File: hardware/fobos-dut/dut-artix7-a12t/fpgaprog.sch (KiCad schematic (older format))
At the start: 6 parts, among them U1 XC7A12T-CSG325

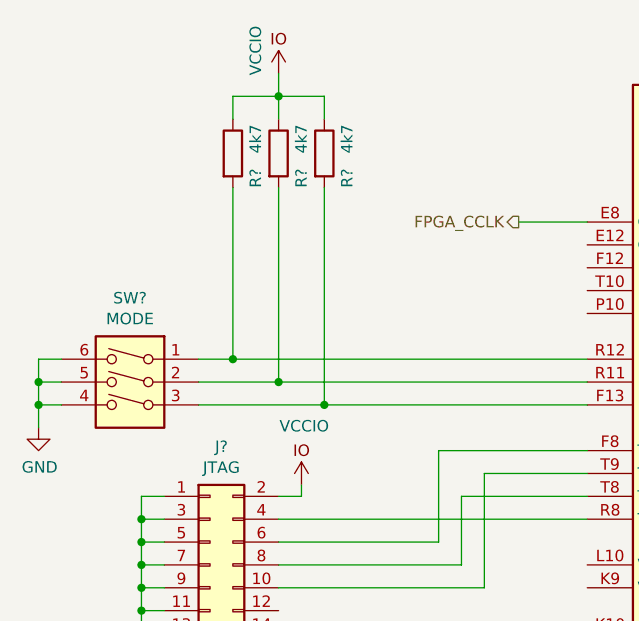
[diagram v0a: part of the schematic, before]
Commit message: artix 7 dut updates
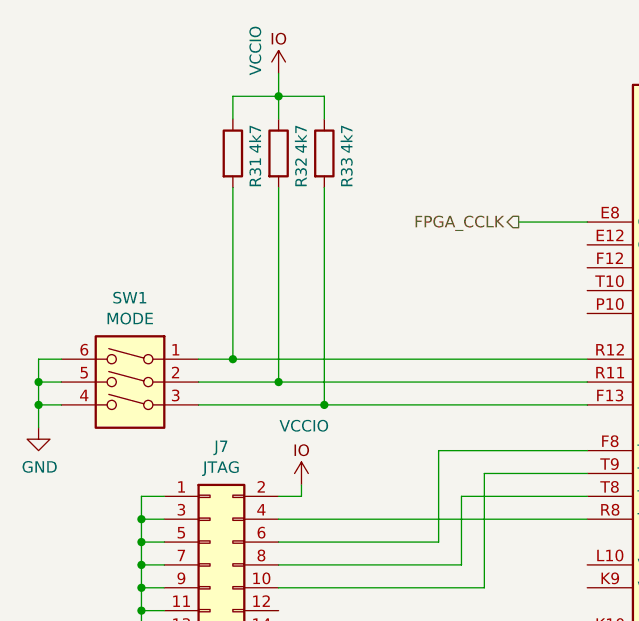
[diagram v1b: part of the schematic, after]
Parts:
- gave numbers to parts that had none: 5
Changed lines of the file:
@@
 $EndBitmap
 $Comp
-L Switch:SW_DIP_x03 SW?
+L Switch:SW_DIP_x03 SW1
 U 1 1 5F5037BE
 P 4500 3200
-F 0 "SW?" H 4500 3667 50  0000 C CNN
+F 0 "SW1" H 4500 3667 50  0000 C CNN
 F 1 "MODE" H 4500 3576 50  0000 C CNN
 F 2 "" H 4500 3200 50  0001 C CNN
@@
 $EndComp
 $Comp
-L power:GND #PWR?
+L power:GND #PWR0129
 U 1 1 5F505FAD
 P 4100 3300
-F 0 "#PWR?" H 4100 3050 50  0001 C CNN
+F 0 "#PWR0129" H 4100 3050 50  0001 C CNN
 F 1 "GND" H 4105 3127 50  0000 C CNN
 F 2 "" H 4100 3300 50  0001 C CNN
@@
 	4800 3200 5350 3200
 $Comp
-L Device:R R?
+L Device:R R33
 U 1 1 5F5112B7
 P 5350 2100
-F 0 "R?" V 5450 1950 50  0000 L CNN
+F 0 "R33" V 5450 1950 50  0000 L CNN
 F 1 "4k7" V 5450 2100 50  0000 L CNN
 F 2 "Resistor_SMD:R_0603_1608Metric" V 5280 2100 50  0001 C CNN
@@
 $EndComp
 $Comp
-L Device:R R?
+L Device:R R32
 U 1 1 5F518AC2
 P 5150 2100
-F 0 "R?" V 5250 1950 50  0000 L CNN
+F 0 "R32" V 5250 1950 50  0000 L CNN
 F 1 "4k7" V 5250 2100 50  0000 L CNN
 F 2 "Resistor_SMD:R_0603_1608Metric" V 5080 2100 50  0001 C CNN
@@
 $EndComp
 $Comp
-L Device:R R?
+L Device:R R31
 U 1 1 5F518EEF
 P 4950 2100
-F 0 "R?" V 5050 1950 50  0000 L CNN
+F 0 "R31" V 5050 1950 50  0000 L CNN
 F 1 "4k7" V 5050 2100 50  0000 L CNN
 F 2 "Resistor_SMD:R_0603_1608Metric" V 4880 2100 50  0001 C CNN
@@
 Connection ~ 5150 1850
 $Comp
-L cerg:VCCIO #PWR?
+L cerg:VCCIO #PWR0130
 U 1 1 5F520C1F
 P 5150 1750
-F 0 "#PWR?" H 5150 1600 50  0001 C CNN
+F 0 "#PWR0130" H 5150 1600 50  0001 C CNN
 F 1 "VCCIO" V 5050 1850 50  0000 C CNN
 F 2 "" H 5150 1750 50  0001 C CNN
@@
 	5150 1750 5150 1850
 $Comp
-L Connector_Generic:Conn_02x07_Odd_Even J?
+L Connector_Generic:Conn_02x07_Odd_Even J7
 U 1 1 5F5293C6
 P 4850 3900
-F 0 "J?" H 4900 4417 50  0000 C CNN
+F 0 "J7" H 4900 4417 50  0000 C CNN
 F 1 "JTAG" H 4900 4326 50  0000 C CNN
 F 2 "" H 4850 3900 50  0001 C CNN
@@
 $EndComp
 $Comp
-L power:GND #PWR?
+L power:GND #PWR0131
 U 1 1 5F52AC29
 P 4550 4350
-F 0 "#PWR?" H 4550 4100 50  0001 C CNN
+F 0 "#PWR0131" H 4550 4100 50  0001 C CNN
 F 1 "GND" H 4555 4177 50  0000 C CNN
 F 2 "" H 4550 4350 50  0001 C CNN
@@
 Connection ~ 4550 3700
 $Comp
-L cerg:VCCIO #PWR?
+L cerg:VCCIO #PWR0132
 U 1 1 5F5300B6
 P 5250 3550
-F 0 "#PWR?" H 5250 3400 50  0001 C CNN
+F 0 "#PWR0132" H 5250 3400 50  0001 C CNN
 F 1 "VCCIO" H 5262 3807 50  0000 C CNN
 F 2 "" H 5250 3550 50  0001 C CNN
